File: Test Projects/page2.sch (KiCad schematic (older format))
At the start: 31 parts, among them P100 SPI_MOSI, P101 SPI_MISO, P102 SPI_SCK, P3 COLS0, P32 PIN8, P33 SIO2, P34 ~HOLD~/SIO3, P35 PIN37, P37 PIN31, P4 COLS1, U3 Teensy_3.2, U32 SPI_MEMORY_SOIC8, U6 SF-MicroSD-12term, U7 SF-74HC595, U8 SF-74HC595

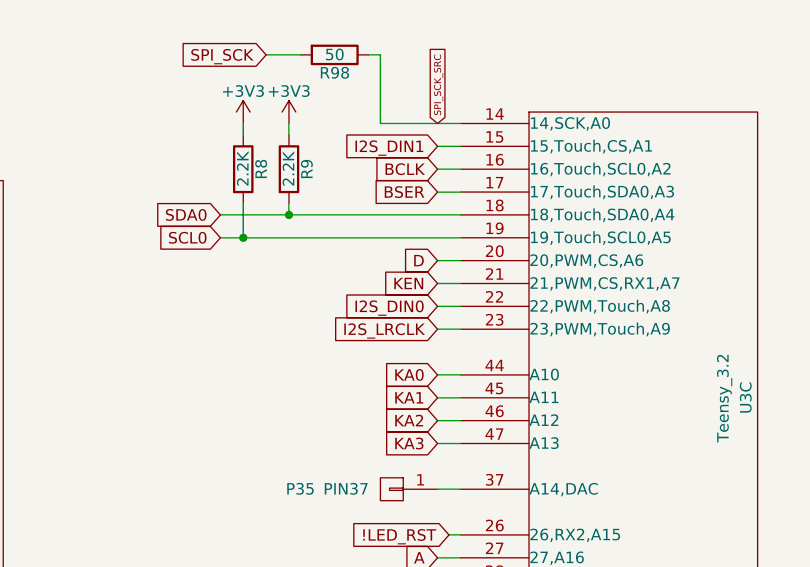
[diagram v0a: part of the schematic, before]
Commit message: went to production
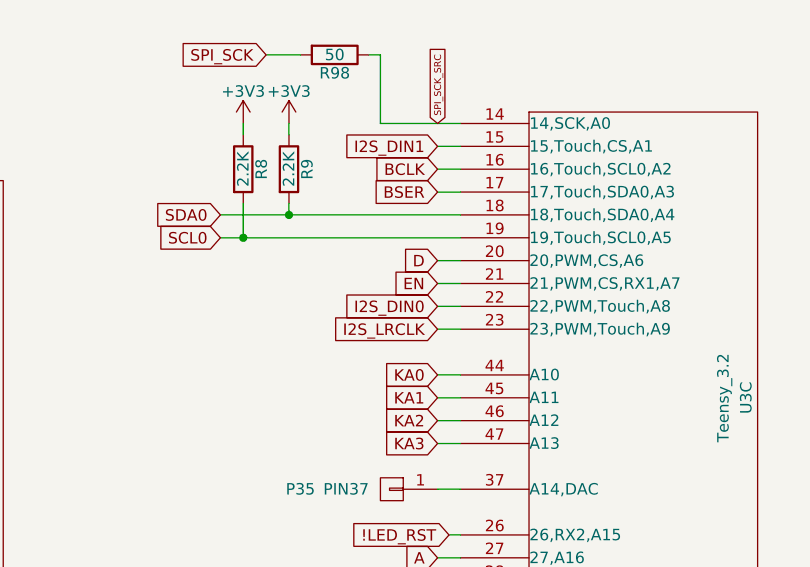
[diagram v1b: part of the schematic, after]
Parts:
- U3: footprint teensy footprints:Teensy_3.2_Route -> teensy footprints:Teensy_3.2_Grid
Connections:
- net KEN renamed EN
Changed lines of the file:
@@
 F 0 "U3" V 7050 2800 50  0000 C CNN
 F 1 "Teensy_3.2" V 6950 2800 50  0000 C CNN
-F 2 "teensy footprints:Teensy_3.2_Route" H 6300 3100 50  0001 C CNN
+F 2 "teensy footprints:Teensy_3.2_Grid" H 6300 3100 50  0001 C CNN
 F 3 "" H 6300 3100 50  0000 C CNN
 	2    6600 2800
@@
 F 0 "U3" V 10350 2750 50  0000 C CNN
 F 1 "Teensy_3.2" V 10250 2750 50  0000 C CNN
-F 2 "teensy footprints:Teensy_3.2_Route" H 9600 3050 50  0001 C CNN
+F 2 "teensy footprints:Teensy_3.2_Grid" H 9600 3050 50  0001 C CNN
 F 3 "" H 9600 3050 50  0000 C CNN
 	3    9900 2750
@@
 BSER
 Text GLabel 9000 2250 0    50   Input ~ 0
-KEN
+EN
 Text GLabel 5700 2950 0    50   Input ~ 0
 I2S_MCLK
@@
 SPI_MOSI
 $Comp
-L +3V3 #PWR024
+L +3V3 #PWR025
 U 1 1 568C434E
 P 8350 1550
-F 0 "#PWR024" H 8350 1400 50  0001 C CNN
+F 0 "#PWR025" H 8350 1400 50  0001 C CNN
 F 1 "+3V3" H 8350 1690 50  0000 C CNN
 F 2 "" H 8350 1550 50  0000 C CNN
@@
 $EndComp
 $Comp
-L +3V3 #PWR025
+L +3V3 #PWR026
 U 1 1 568C4354
 P 8150 1550
-F 0 "#PWR025" H 8150 1400 50  0001 C CNN
+F 0 "#PWR026" H 8150 1400 50  0001 C CNN
 F 1 "+3V3" H 8150 1690 50  0000 C CNN
 F 2 "" H 8150 1550 50  0000 C CNN
@@
 $EndComp
 $Comp
-L GND #PWR026
+L GND #PWR027
 U 1 1 56A0F405
 P 3750 1950
-F 0 "#PWR026" H 3750 1700 50  0001 C CNN
+F 0 "#PWR027" H 3750 1700 50  0001 C CNN
 F 1 "GND" H 3750 1800 50  0000 C CNN
 F 2 "" H 3750 1950 50  0000 C CNN
@@
 $EndComp
 $Comp
-L GND #PWR027
+L GND #PWR028
 U 1 1 56A0F6ED
 P 3500 3750
-F 0 "#PWR027" H 3500 3500 50  0001 C CNN
+F 0 "#PWR028" H 3500 3500 50  0001 C CNN
 F 1 "GND" H 3500 3600 50  0000 C CNN
 F 2 "" H 3500 3750 50  0000 C CNN
@@
 $EndComp
 $Comp
-L GND #PWR028
+L GND #PWR029
 U 1 1 56A0FB18
 P 2700 7400
-F 0 "#PWR028" H 2700 7150 50  0001 C CNN
+F 0 "#PWR029" H 2700 7150 50  0001 C CNN
 F 1 "GND" H 2700 7250 50  0000 C CNN
 F 2 "" H 2700 7400 50  0000 C CNN
@@
 $EndComp
 $Comp
-L GND #PWR029
+L GND #PWR030
 U 1 1 56A0FBC8
 P 5200 7400
-F 0 "#PWR029" H 5200 7150 50  0001 C CNN
+F 0 "#PWR030" H 5200 7150 50  0001 C CNN
 F 1 "GND" H 5200 7250 50  0000 C CNN
 F 2 "" H 5200 7400 50  0000 C CNN
@@
 $EndComp
 $Comp
-L +3V3 #PWR030
+L +3V3 #PWR031
 U 1 1 56A0FE25
 P 3500 1400
-F 0 "#PWR030" H 3500 1250 50  0001 C CNN
+F 0 "#PWR031" H 3500 1250 50  0001 C CNN
 F 1 "+3V3" H 3500 1540 50  0000 C CNN
 F 2 "" H 3500 1400 50  0000 C CNN
@@
 $EndComp
 $Comp
-L +3V3 #PWR031
+L +3V3 #PWR032
 U 1 1 56A104A5
 P 2700 6300
-F 0 "#PWR031" H 2700 6150 50  0001 C CNN
+F 0 "#PWR032" H 2700 6150 50  0001 C CNN
 F 1 "+3V3" H 2700 6440 50  0000 C CNN
 F 2 "" H 2700 6300 50  0000 C CNN
@@
 $EndComp
 $Comp
-L +3V3 #PWR032
+L +3V3 #PWR033
 U 1 1 56A105FA
 P 5200 6300
-F 0 "#PWR032" H 5200 6150 50  0001 C CNN
+F 0 "#PWR033" H 5200 6150 50  0001 C CNN
 F 1 "+3V3" H 5200 6440 50  0000 C CNN
 F 2 "" H 5200 6300 50  0000 C CNN
@@
 SPI_MISO
 $Comp
-L +3V3 #PWR033
+L +3V3 #PWR034
 U 1 1 56A12235
 P 2150 2000
-F 0 "#PWR033" H 2150 1850 50  0001 C CNN
+F 0 "#PWR034" H 2150 1850 50  0001 C CNN
 F 1 "+3V3" H 2150 2140 50  0000 C CNN
 F 2 "" H 2150 2000 50  0000 C CNN
@@
 $EndComp
 $Comp
-L +3V3 #PWR034
+L +3V3 #PWR035
 U 1 1 56A12282
 P 1950 2000
-F 0 "#PWR034" H 1950 1850 50  0001 C CNN
+F 0 "#PWR035" H 1950 1850 50  0001 C CNN
 F 1 "+3V3" H 1950 2140 50  0000 C CNN
 F 2 "" H 1950 2000 50  0000 C CNN
@@
 $EndComp
 $Comp
-L +3V3 #PWR035
+L +3V3 #PWR036
 U 1 1 56A16EA5
 P 1200 4850
-F 0 "#PWR035" H 1200 4700 50  0001 C CNN
+F 0 "#PWR036" H 1200 4700 50  0001 C CNN
 F 1 "+3V3" H 1200 4990 50  0000 C CNN
 F 2 "" H 1200 4850 50  0000 C CNN
@@
 $EndComp
 $Comp
-L +3V3 #PWR036
+L +3V3 #PWR037
 U 1 1 56A16EFE
 P 3750 4800
-F 0 "#PWR036" H 3750 4650 50  0001 C CNN
+F 0 "#PWR037" H 3750 4650 50  0001 C CNN
 F 1 "+3V3" H 3750 4940 50  0000 C CNN
 F 2 "" H 3750 4800 50  0000 C CNN
@@
 $EndComp
 $Comp
-L GND #PWR037
+L GND #PWR038
 U 1 1 56B2615C
 P 4900 3700
-F 0 "#PWR037" H 4900 3450 50  0001 C CNN
+F 0 "#PWR038" H 4900 3450 50  0001 C CNN
 F 1 "GND" H 4900 3550 50  0000 C CNN
 F 2 "" H 4900 3700 50  0000 C CNN
@@
 $EndComp
 $Comp
-L GND #PWR038
+L GND #PWR039
 U 1 1 56B26162
 P 2300 4000
-F 0 "#PWR038" H 2300 3750 50  0001 C CNN
+F 0 "#PWR039" H 2300 3750 50  0001 C CNN
 F 1 "GND" H 2300 3850 50  0000 C CNN
 F 2 "" H 2300 4000 50  0000 C CNN
@@
 $EndComp
 $Comp
-L GND #PWR039
+L GND #PWR040
 U 1 1 56B26168
 P 2650 4000
-F 0 "#PWR039" H 2650 3750 50  0001 C CNN
+F 0 "#PWR040" H 2650 3750 50  0001 C CNN
 F 1 "GND" H 2650 3850 50  0000 C CNN
 F 2 "" H 2650 4000 50  0000 C CNN
@@
 $EndComp
 $Comp
-L +3V3 #PWR040
+L +3V3 #PWR041
 U 1 1 56B12EEC
 P 7850 4750
-F 0 "#PWR040" H 7850 4600 50  0001 C CNN
+F 0 "#PWR041" H 7850 4600 50  0001 C CNN
 F 1 "+3V3" H 7850 4890 50  0000 C CNN
 F 2 "" H 7850 4750 50  0000 C CNN
@@
 $EndComp
 $Comp
-L +3V3 #PWR041
+L +3V3 #PWR042
 U 1 1 56B12EF2
 P 7650 4750
-F 0 "#PWR041" H 7650 4600 50  0001 C CNN
+F 0 "#PWR042" H 7650 4600 50  0001 C CNN
 F 1 "+3V3" H 7650 4890 50  0000 C CNN
 F 2 "" H 7650 4750 50  0000 C CNN
